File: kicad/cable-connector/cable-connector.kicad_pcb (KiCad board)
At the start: 2 copper layers, 92 x 69 mm, 11 parts

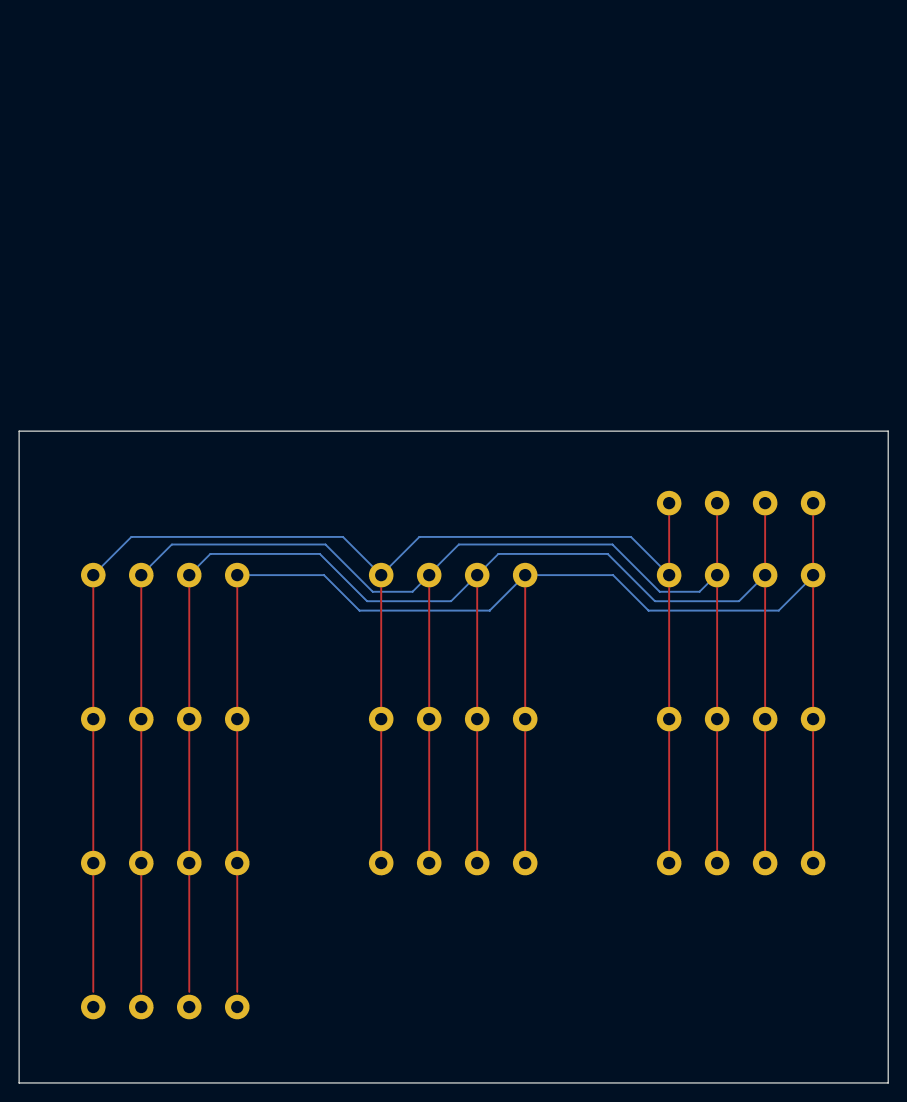
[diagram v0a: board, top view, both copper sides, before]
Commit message: Dreamworker
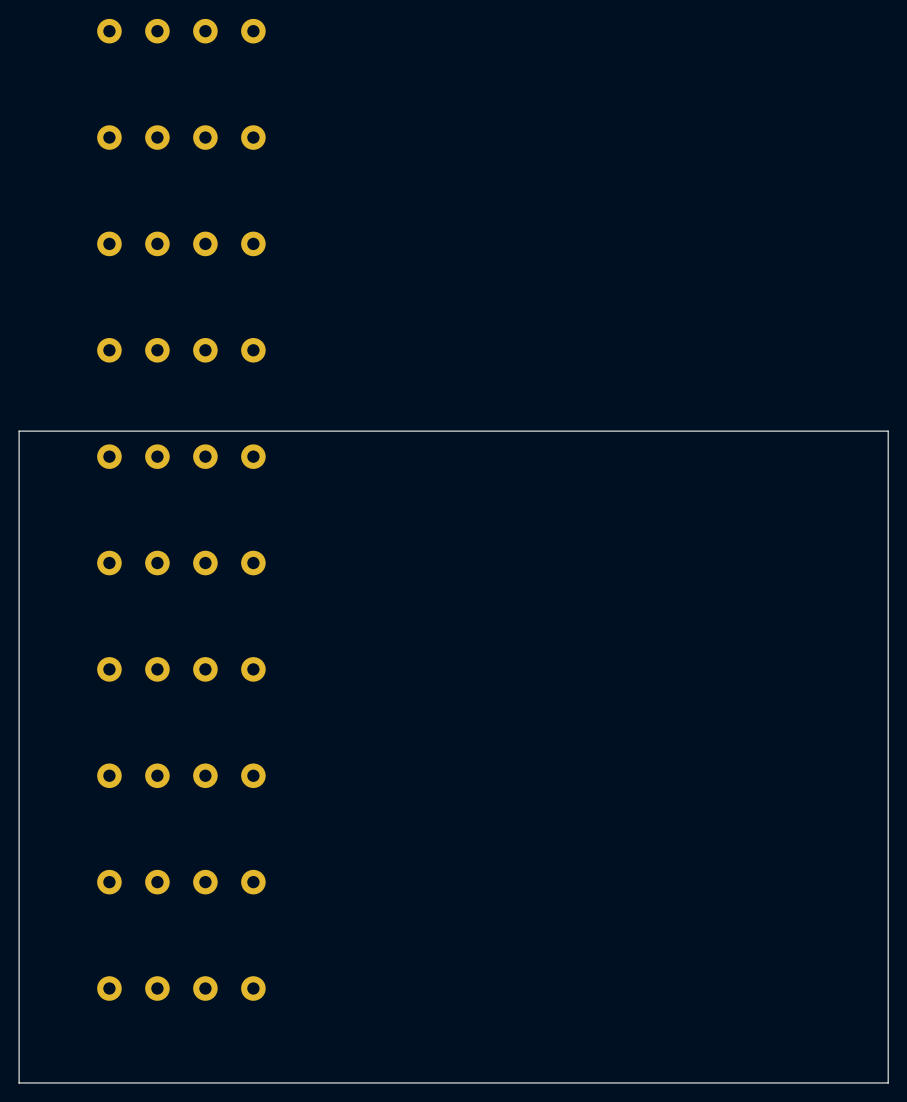
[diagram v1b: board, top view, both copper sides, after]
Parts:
- removed REF** (x11): SDI_Connector, footprints:SDI_Connector
- added J1: Conn_01x04_Pin, footprints:SDI_Connector, F.Cu at (92.2, 22.7)
- added J10: Conn_01x04_Pin, footprints:SDI_Connector, F.Cu at (92.2, 124.0)
- added J2: Conn_01x04_Pin, footprints:SDI_Connector, F.Cu at (92.2, 33.9)
- added J3: Conn_01x04_Pin, footprints:SDI_Connector, F.Cu at (92.2, 45.2)
- added J4: Conn_01x04_Pin, footprints:SDI_Connector, F.Cu at (92.2, 56.4)
- added J5: Conn_01x04_Pin, footprints:SDI_Connector, F.Cu at (92.2, 67.7)
- added J6: Conn_01x04_Pin, footprints:SDI_Connector, F.Cu at (92.2, 79.0)
- added J7: Conn_01x04_Pin, footprints:SDI_Connector, F.Cu at (92.2, 90.2)
- added J8: Conn_01x04_Pin, footprints:SDI_Connector, F.Cu at (92.2, 101.5)
- added J9: Conn_01x04_Pin, footprints:SDI_Connector, F.Cu at (92.2, 112.7)
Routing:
- net (no net): track 724.1 -> 0.00 mm

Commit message: Cradle of Hope
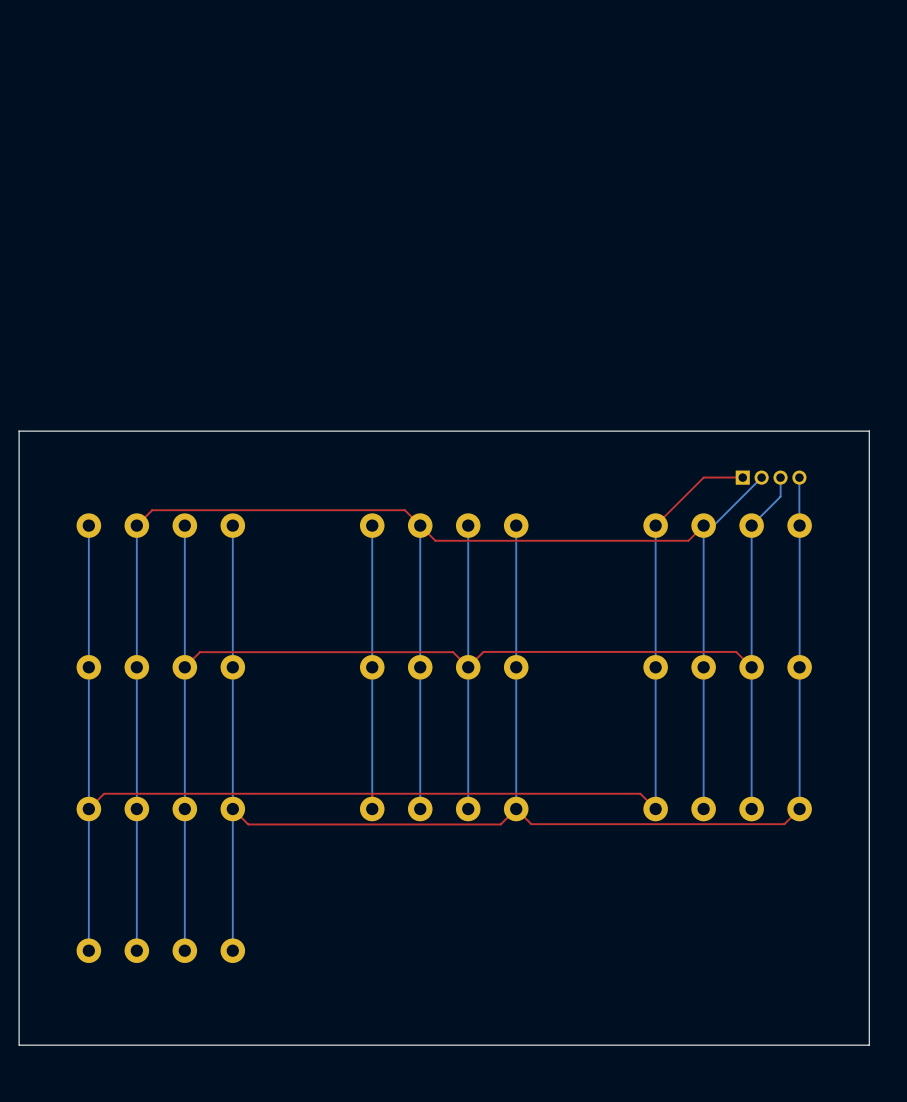
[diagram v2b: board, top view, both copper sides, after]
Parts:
- added J11: Conn_01x04_Pin, footprints:GROVE-HW4-2.0, B.Cu at (154.6, 69.9)
- moved J4 63.6 mm to (90.0, 120.0)
- moved J8 63.6 mm to (150.0, 75.0)
- moved J9 62.1 mm to (150.0, 90.0)
- moved J10 60.9 mm to (150.0, 105.0)
- moved J3 59.9 mm to (90.0, 105.0)
- moved J2 56.1 mm to (90.0, 90.0)
- moved J1 52.4 mm to (90.0, 75.0)
- moved J7 31.5 mm to (120.0, 105.0)
- moved J6 29.9 mm to (120.0, 90.0)
- moved J5 28.8 mm to (120.0, 75.0)
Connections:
- J1 pad 1: unconnected-(J1-Pin_1-Pad1) -> /BLUE
- J1 pad 2: unconnected-(J1-Pin_2-Pad2) -> /WHITE
- J1 pad 3: unconnected-(J1-Pin_3-Pad3) -> /BROWN
- J1 pad 4: unconnected-(J1-Pin_4-Pad4) -> /BLACK
- J10 pad 1: unconnected-(J10-Pin_1-Pad1) -> /BLUE
- J10 pad 2: unconnected-(J10-Pin_2-Pad2) -> /WHITE
- J10 pad 3: unconnected-(J10-Pin_3-Pad3) -> /BROWN
- J10 pad 4: unconnected-(J10-Pin_4-Pad4) -> /BLACK
- J2 pad 1: unconnected-(J2-Pin_1-Pad1) -> /BLUE
- J2 pad 2: unconnected-(J2-Pin_2-Pad2) -> /WHITE
- J2 pad 3: unconnected-(J2-Pin_3-Pad3) -> /BROWN
- J2 pad 4: unconnected-(J2-Pin_4-Pad4) -> /BLACK
- J3 pad 1: unconnected-(J3-Pin_1-Pad1) -> /BLUE
- J3 pad 2: unconnected-(J3-Pin_2-Pad2) -> /WHITE
- J3 pad 3: unconnected-(J3-Pin_3-Pad3) -> /BROWN
- J3 pad 4: unconnected-(J3-Pin_4-Pad4) -> /BLACK
- J4 pad 1: unconnected-(J4-Pin_1-Pad1) -> /BLUE
- J4 pad 2: unconnected-(J4-Pin_2-Pad2) -> /WHITE
- J4 pad 3: unconnected-(J4-Pin_3-Pad3) -> /BROWN
- J4 pad 4: unconnected-(J4-Pin_4-Pad4) -> /BLACK
- J5 pad 1: unconnected-(J5-Pin_1-Pad1) -> /BLUE
- J5 pad 2: unconnected-(J5-Pin_2-Pad2) -> /WHITE
- J5 pad 3: unconnected-(J5-Pin_3-Pad3) -> /BROWN
- J5 pad 4: unconnected-(J5-Pin_4-Pad4) -> /BLACK
- J6 pad 1: unconnected-(J6-Pin_1-Pad1) -> /BLUE
- J6 pad 2: unconnected-(J6-Pin_2-Pad2) -> /WHITE
- J6 pad 3: unconnected-(J6-Pin_3-Pad3) -> /BROWN
- J6 pad 4: unconnected-(J6-Pin_4-Pad4) -> /BLACK
- J7 pad 1: unconnected-(J7-Pin_1-Pad1) -> /BLUE
- J7 pad 2: unconnected-(J7-Pin_2-Pad2) -> /WHITE
- J7 pad 3: unconnected-(J7-Pin_3-Pad3) -> /BROWN
- J7 pad 4: unconnected-(J7-Pin_4-Pad4) -> /BLACK
- J8 pad 1: unconnected-(J8-Pin_1-Pad1) -> /BLUE
- J8 pad 2: unconnected-(J8-Pin_2-Pad2) -> /WHITE
- J8 pad 3: unconnected-(J8-Pin_3-Pad3) -> /BROWN
- J8 pad 4: unconnected-(J8-Pin_4-Pad4) -> /BLACK
- J9 pad 1: unconnected-(J9-Pin_1-Pad1) -> /BLUE
- J9 pad 2: unconnected-(J9-Pin_2-Pad2) -> /WHITE
- J9 pad 3: unconnected-(J9-Pin_3-Pad3) -> /BROWN
- J9 pad 4: unconnected-(J9-Pin_4-Pad4) -> /BLACK
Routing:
- net /BLUE: track 0.00 -> 179.3 mm
- net /WHITE: track 0.00 -> 175.9 mm
- net /BROWN: track 0.00 -> 174.0 mm
- net /BLACK: track 0.00 -> 172.8 mm
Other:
- board size 92 x 69 mm -> 90 x 65 mm
